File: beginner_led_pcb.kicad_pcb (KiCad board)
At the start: 2 copper layers, 58.5 x 14.5 mm, 30 parts, among them J1 Conn_01x03_Pin

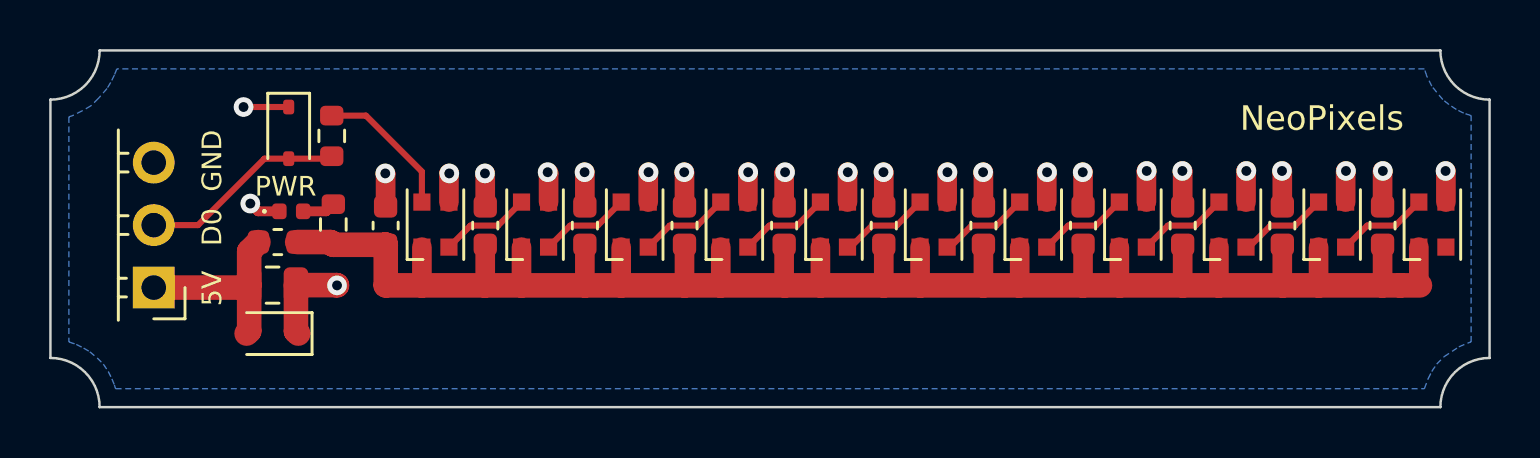
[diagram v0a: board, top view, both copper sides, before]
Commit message: gerber files
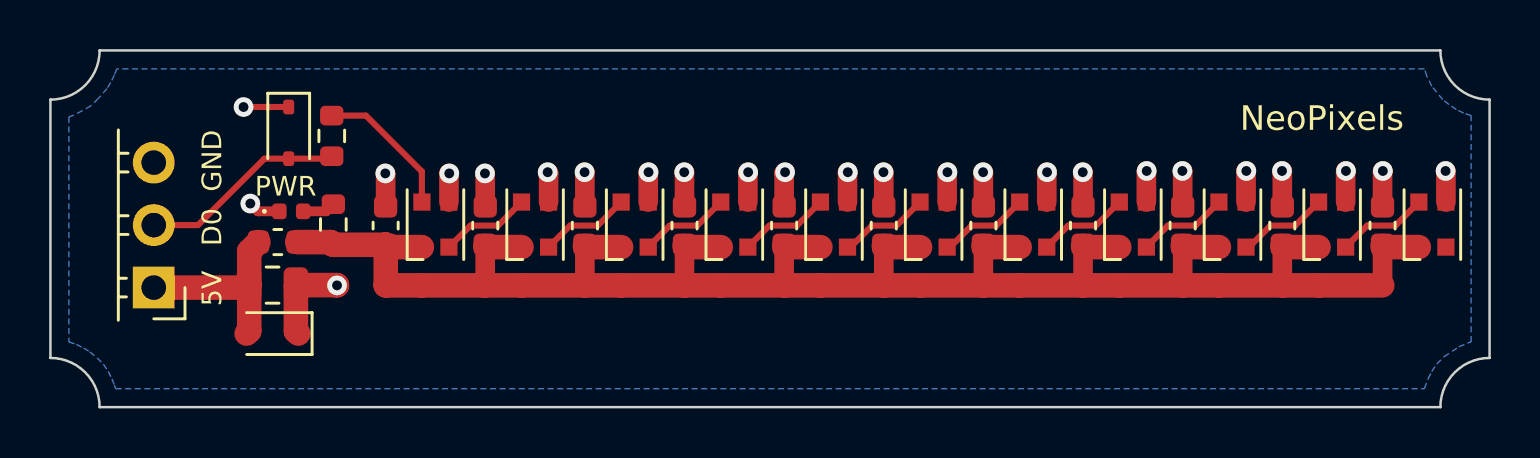
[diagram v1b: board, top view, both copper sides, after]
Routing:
- net +5V: track 81.1 -> 78.9 mm
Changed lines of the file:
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@@
   (segment (start 212.175 111.395) (end 212.175 113.035) (width 0.8) (layer "F.Cu") (net 1))
   (segment (start 216.225 113.045) (end 216.23 113.05) (width 0.8) (layer "F.Cu") (net 1))
+  (segment (start 213.65 111.495) (end 212.225 111.495) (width 1) (layer "F.Cu") (net 1))
+  (segment (start 208.225 111.495) (end 208.125 111.395) (width 1) (layer "F.Cu") (net 1))
   (segment (start 228.375 111.395) (end 228.375 113.045) (width 0.8) (layer "F.Cu") (net 1))
   (segment (start 208.125 111.395) (end 208.13 111.4) (width 1) (layer "F.Cu") (net 1))
+  (segment (start 240.575 111.495) (end 240.525 111.445) (width 1) (layer "F.Cu") (net 1))
   (segment (start 240.525 111.395) (end 240.525 113.045) (width 0.8) (layer "F.Cu") (net 1))
-  (segment (start 249.37 113.05) (end 250.17 113.05) (width 1) (layer "F.Cu") (net 1))
-  (segment (start 229.85 111.495) (end 229.85 113.04) (width 0.8) (layer "F.Cu") (net 1))
+  (segment (start 228.425 111.495) (end 228.375 111.445) (width 1) (layer "F.Cu") (net 1))
   (segment (start 225.81 113.05) (end 228.37 113.05) (width 1) (layer "F.Cu") (net 1))
-  (segment (start 237.95 111.495) (end 237.95 113.03) (width 0.8) (layer "F.Cu") (net 1))
+  (segment (start 212.225 111.495) (end 212.175 111.445) (width 1) (layer "F.Cu") (net 1))
+  (segment (start 248.7 111.495) (end 248.65 111.445) (width 1) (layer "F.Cu") (net 1))
   (segment (start 232.425 111.395) (end 232.425 113.045) (width 0.8) (layer "F.Cu") (net 1))
   (segment (start 224.325 113.025) (end 224.35 113.05) (width 0.8) (layer "F.Cu") (net 1))
+  (segment (start 229.85 111.495) (end 228.425 111.495) (width 1) (layer "F.Cu") (net 1))
   (segment (start 213.65 113.05) (end 216.23 113.05) (width 1) (layer "F.Cu") (net 1))
   (segment (start 232.42 113.05) (end 233.88 113.05) (width 1) (layer "F.Cu") (net 1))
   (segment (start 240.53 113.05) (end 242 113.05) (width 1) (layer "F.Cu") (net 1))
-  (segment (start 209.6 111.495) (end 209.6 113.05) (width 0.8) (layer "F.Cu") (net 1))
-  (segment (start 221.75 111.495) (end 221.75 113.04) (width 0.8) (layer "F.Cu") (net 1))
-  (segment (start 233.9 113.03) (end 233.88 113.05) (width 0.8) (layer "F.Cu") (net 1))
-  (segment (start 246.05 111.495) (end 246.05 113.04) (width 0.8) (layer "F.Cu") (net 1))
+  (segment (start 217.7 111.495) (end 216.275 111.495) (width 1) (layer "F.Cu") (net 1))
   (segment (start 208.12 111.4) (end 208.125 111.395) (width 1) (layer "F.Cu") (net 1))
   (segment (start 229.86 113.05) (end 232.42 113.05) (width 1) (layer "F.Cu") (net 1))
-  (segment (start 242 111.495) (end 242 113.05) (width 0.8) (layer "F.Cu") (net 1))
-  (segment (start 221.75 113.04) (end 221.74 113.05) (width 0.8) (layer "F.Cu") (net 1))
-  (segment (start 250.125 111.495) (end 250.125 113.005) (width 0.8) (layer "F.Cu") (net 1))
-  (segment (start 217.7 111.495) (end 217.7 113.05) (width 0.8) (layer "F.Cu") (net 1))
+  (segment (start 242 111.495) (end 240.575 111.495) (width 1) (layer "F.Cu") (net 1))
+  (segment (start 237.95 111.495) (end 236.525 111.495) (width 1) (layer "F.Cu") (net 1))
   (segment (start 236.475 113.045) (end 236.47 113.05) (width 0.8) (layer "F.Cu") (net 1))
+  (segment (start 232.475 111.495) (end 232.425 111.445) (width 1) (layer "F.Cu") (net 1))
   (segment (start 232.425 113.045) (end 232.42 113.05) (width 0.8) (layer "F.Cu") (net 1))
   (segment (start 208.13 113.05) (end 209.6 113.05) (width 1) (layer "F.Cu") (net 1))
-  (segment (start 237.95 113.03) (end 237.97 113.05) (width 0.8) (layer "F.Cu") (net 1))
   (segment (start 228.37 113.05) (end 229.86 113.05) (width 1) (layer "F.Cu") (net 1))
   (segment (start 236.47 113.05) (end 237.97 113.05) (width 1) (layer "F.Cu") (net 1))
+  (segment (start 221.75 111.495) (end 220.325 111.495) (width 1) (layer "F.Cu") (net 1))
   (segment (start 236.475 111.395) (end 236.475 113.045) (width 0.8) (layer "F.Cu") (net 1))
   (segment (start 206 111.4) (end 208.12 111.4) (width 1) (layer "F.Cu") (net 1))
+  (segment (start 244.625 111.495) (end 244.575 111.445) (width 1) (layer "F.Cu") (net 1))
   (segment (start 240.525 113.045) (end 240.53 113.05) (width 0.8) (layer "F.Cu") (net 1))
   (segment (start 220.275 113.045) (end 220.28 113.05) (width 0.8) (layer "F.Cu") (net 1))
-  (segment (start 225.8 113.04) (end 225.81 113.05) (width 0.8) (layer "F.Cu") (net 1))
   (segment (start 248.65 111.395) (end 248.65 113.04) (width 0.8) (layer "F.Cu") (net 1))
   (segment (start 221.74 113.05) (end 224.35 113.05) (width 1) (layer "F.Cu") (net 1))
-  (segment (start 250.125 113.005) (end 250.17 113.05) (width 0.8) (layer "F.Cu") (net 1))
   (segment (start 228.375 113.045) (end 228.37 113.05) (width 0.8) (layer "F.Cu") (net 1))
   (segment (start 248.65 113.04) (end 248.64 113.05) (width 0.8) (layer "F.Cu") (net 1))
+  (segment (start 220.325 111.495) (end 220.275 111.445) (width 1) (layer "F.Cu") (net 1))
   (segment (start 246.06 113.05) (end 248.64 113.05) (width 1) (layer "F.Cu") (net 1))
+  (segment (start 250.125 111.495) (end 248.7 111.495) (width 1) (layer "F.Cu") (net 1))
   (segment (start 212.16 113.05) (end 213.65 113.05) (width 1) (layer "F.Cu") (net 1))
   (segment (start 216.23 113.05) (end 217.7 113.05) (width 1) (layer "F.Cu") (net 1))
+  (segment (start 209.6 111.495) (end 208.225 111.495) (width 1) (layer "F.Cu") (net 1))
   (segment (start 204.53 111.29) (end 205.89 111.29) (width 1) (layer "F.Cu") (net 1))
+  (segment (start 224.375 111.495) (end 224.325 111.445) (width 1) (layer "F.Cu") (net 1))
+  (segment (start 216.275 111.495) (end 216.225 111.445) (width 1) (layer "F.Cu") (net 1))
   (segment (start 244.575 111.395) (end 244.575 113.035) (width 0.8) (layer "F.Cu") (net 1))
+  (segment (start 246.05 111.495) (end 244.625 111.495) (width 1) (layer "F.Cu") (net 1))
   (segment (start 242 113.05) (end 244.59 113.05) (width 1) (layer "F.Cu") (net 1))
   (segment (start 244.59 113.05) (end 246.06 113.05) (width 1) (layer "F.Cu") (net 1))
-  (segment (start 229.85 113.04) (end 229.86 113.05) (width 0.8) (layer "F.Cu") (net 1))
-  (segment (start 233.9 111.495) (end 233.9 113.03) (width 0.8) (layer "F.Cu") (net 1))
   (segment (start 224.325 111.395) (end 224.325 113.025) (width 0.8) (layer "F.Cu") (net 1))
-  (segment (start 213.65 111.495) (end 213.65 113.05) (width 0.8) (layer "F.Cu") (net 1))
+  (segment (start 236.525 111.495) (end 236.475 111.445) (width 1) (layer "F.Cu") (net 1))
   (segment (start 209.6 113.05) (end 212.16 113.05) (width 1) (layer "F.Cu") (net 1))
-  (segment (start 248.64 113.05) (end 249.37 113.05) (width 1) (layer "F.Cu") (net 1))
   (segment (start 233.88 113.05) (end 236.47 113.05) (width 1) (layer "F.Cu") (net 1))
-  (segment (start 225.8 111.495) (end 225.8 113.04) (width 0.8) (layer "F.Cu") (net 1))
   (segment (start 224.35 113.05) (end 225.81 113.05) (width 1) (layer "F.Cu") (net 1))
   (segment (start 237.97 113.05) (end 240.53 113.05) (width 1) (layer "F.Cu") (net 1))
@@
   (segment (start 212.175 113.035) (end 212.16 113.05) (width 0.8) (layer "F.Cu") (net 1))
   (segment (start 217.7 113.05) (end 220.28 113.05) (width 1) (layer "F.Cu") (net 1))
-  (segment (start 246.05 113.04) (end 246.06 113.05) (width 0.8) (layer "F.Cu") (net 1))
   (segment (start 244.575 113.035) (end 244.59 113.05) (width 0.8) (layer "F.Cu") (net 1))
+  (segment (start 233.9 111.495) (end 232.475 111.495) (width 1) (layer "F.Cu") (net 1))
+  (segment (start 225.8 111.495) (end 224.375 111.495) (width 1) (layer "F.Cu") (net 1))
   (segment (start 222.85 108.4625) (end 222.8625 108.45) (width 0.8) (layer "F.Cu") (net 2))
   (segment (start 203.805 110.04) (end 202.94 110.04) (width 0.4) (layer "F.Cu") (net 2))
